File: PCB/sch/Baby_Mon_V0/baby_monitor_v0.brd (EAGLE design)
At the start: 20 x 20 mm, 37 parts, among them J1 BATT-COIN1CR1216, U1 NRF5340-QKAA-AB0-R, U2 MAX30101EFD+, U3 MAX30205MTA+, X1 XRCGB32M000F2P10R0

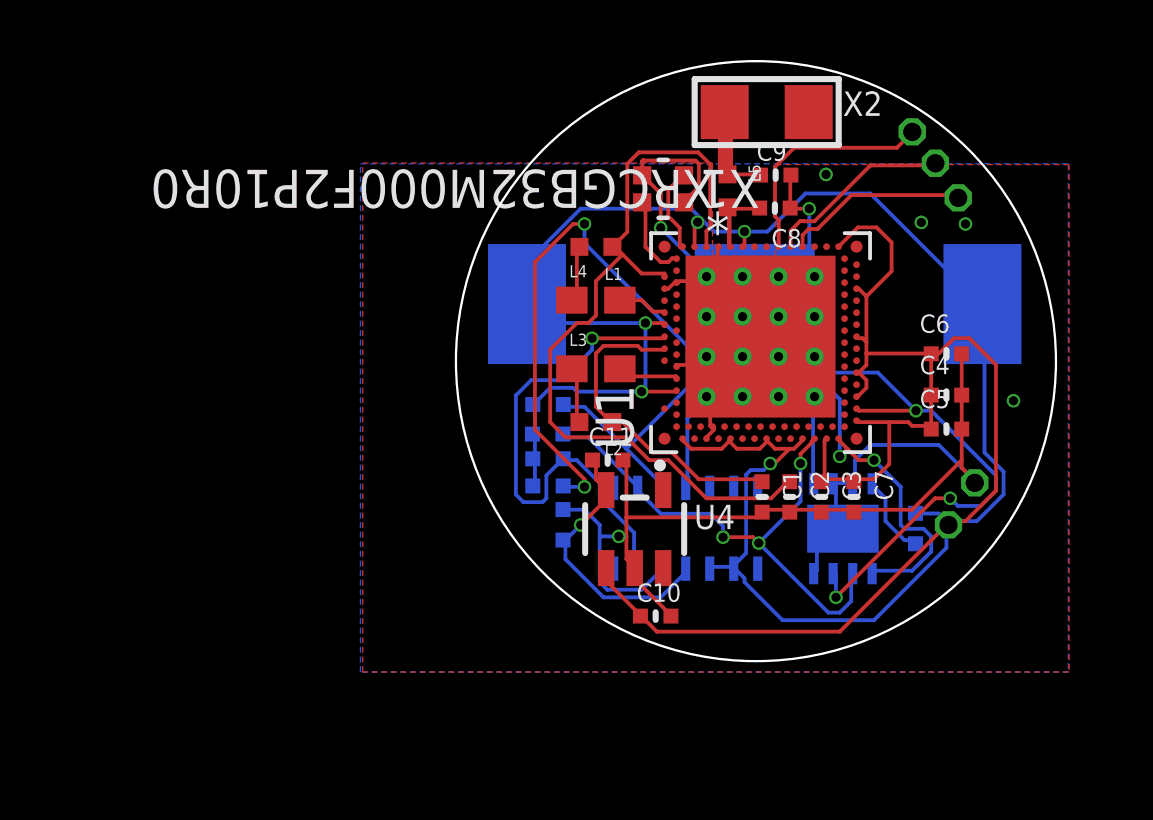
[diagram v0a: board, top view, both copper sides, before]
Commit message: u
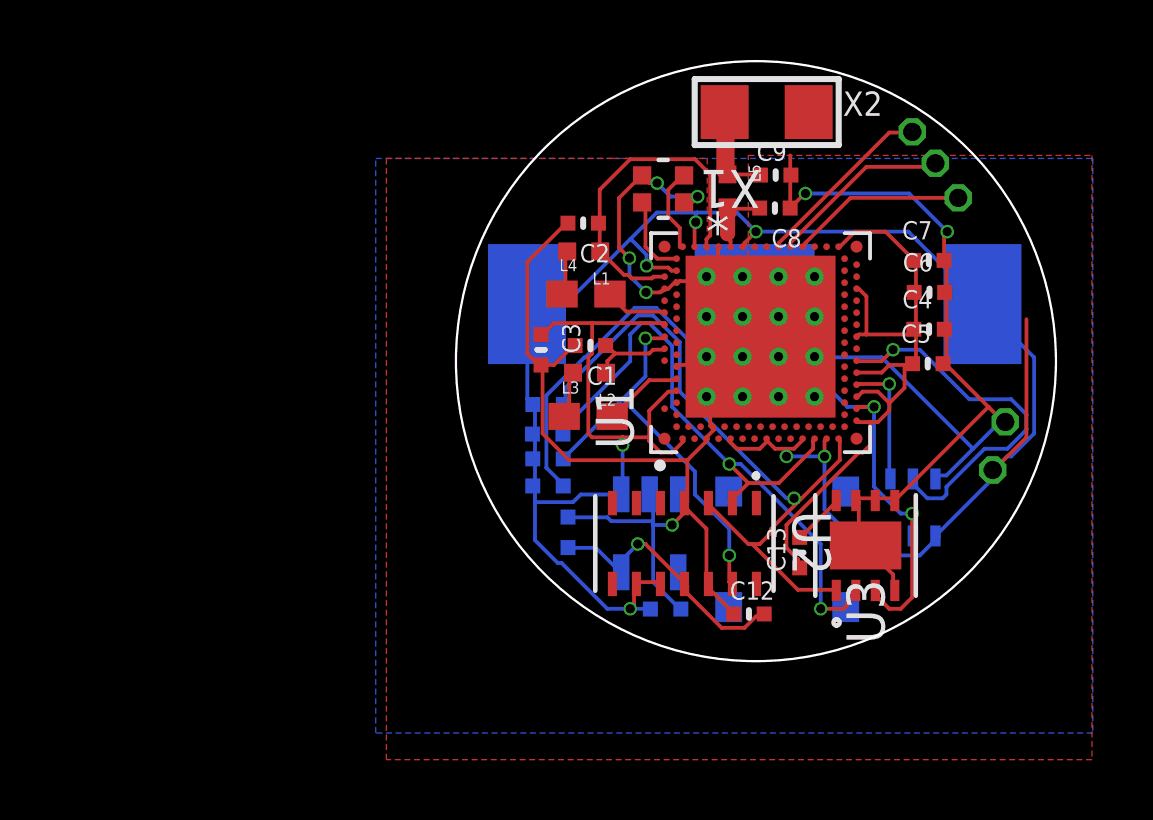
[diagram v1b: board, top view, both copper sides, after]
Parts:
- added SW2: (no value), graftel-internal-ic:MICROBUILDER_BTN_EVQPQ_4.5MM
- added U$2: (no value), graftel-internal-ic:MICROBUILDER_APA102_2020
- moved C2 11.4 mm to (0.08, 14.0), turned to 180 degrees
- moved C3 10.6 mm to (-1.32, 9.77)
- moved C7 8.27 mm to (11.6, 12.8), turned to 0 degrees
- moved C1 7.63 mm to (0.32, 9.92), turned to 180 degrees
- moved C12 6.87 mm to (5.61, 0.97), flipped to the top, turned to 0 degrees
- moved C13 3.94 mm to (7.30, 3.02), flipped to the top, turned to 90 degrees
- moved C11 2.75 mm to (-0.42, 3.69), flipped to the bottom, turned to 90 degrees
- moved J8 2.35 mm to (13.7, 5.77)
- moved J7 2.27 mm to (14.2, 7.37)
- moved C4 2.27 mm to (11.6, 10.5)
- moved C5 2.27 mm to (11.6, 9.31)
- moved C6 2.12 mm to (11.6, 11.7)
- moved L2 1.66 mm to (0.29, 9.01)
- moved L3 1.61 mm to (0.25, 7.55)
- moved U3 0.94 mm to (9.50, 3.25), flipped to the top
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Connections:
- new net CI: U$2.5, U1.AL13
- new net DI: U$2.6, U1.AL9
- net 3.3V: now also U$2.3
- net GND: now also U$2.4
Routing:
- net N$8: track 27.1 -> 11.4 mm
- net GND: track 95.8 -> 110.9 mm, vias 6 -> 7
- net OS: track 39.4 -> 26.7 mm, vias 5 -> 2
- net CI: track 0.00 -> 12.5 mm, vias 0 -> 1
- net N$9: track 10.8 -> 2.94 mm
- net 3.3V: track 112.1 -> 105.8 mm, vias 5 -> 7
- net SCL: track 17.7 -> 23.6 mm, vias 3 -> 2
- net DI: track 0.00 -> 4.26 mm, vias 0 -> 1
- net INT: track 17.1 -> 13.5 mm, vias 1 -> 2
- net N$2: track 7.80 -> 6.13 mm
- net N$14: track 2.74 -> 1.74 mm
- net N$7: track 2.05 -> 2.68 mm
- net SDA: vias 2 -> 1
